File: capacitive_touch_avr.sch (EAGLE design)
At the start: 10 parts, among them J2 JACK-2.1MM

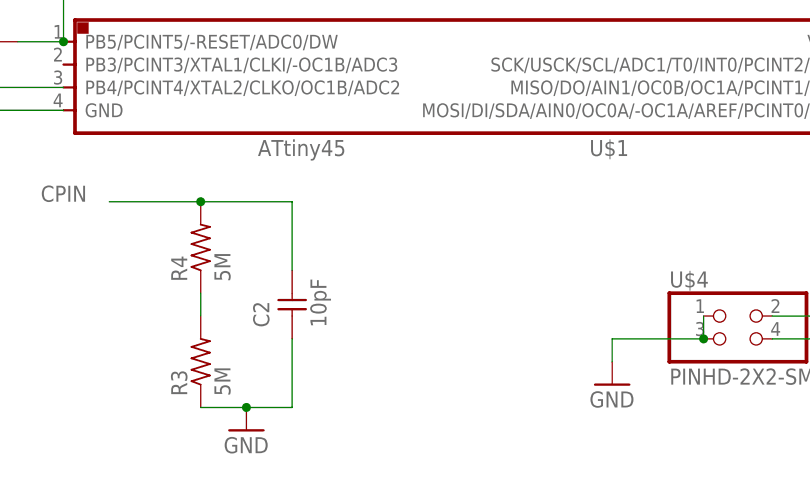
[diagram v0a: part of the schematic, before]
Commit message: Version 1. Touch pad + full wiring
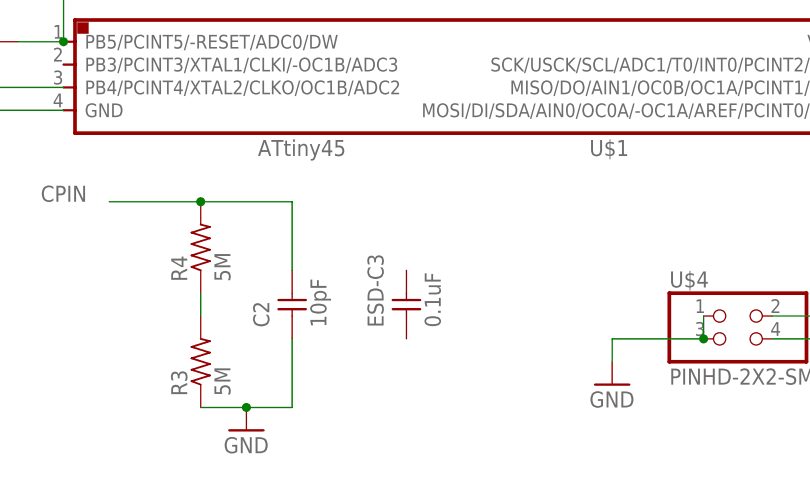
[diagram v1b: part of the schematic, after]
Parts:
- added ESD-C3: 0.1uF, fab:CAP-UNPOLARIZEDFAB
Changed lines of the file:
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@@
 <part name="P+7" library="supply1" library_urn="urn:adsk.eagle:library:371" deviceset="VCC" device=""/>
 <part name="J2" library="fab" deviceset="JACK-2.1MM" device=""/>
+<part name="ESD-C3" library="fab" deviceset="CAP-UNPOLARIZED" device="FAB" value="0.1uF"/>
 </parts>
 <sheets>
@@
 <instance part="P+7" gate="VCC" x="25.4" y="58.42" rot="R180"/>
 <instance part="J2" gate="G$1" x="27.94" y="73.66" rot="R90"/>
+<instance part="ESD-C3" gate="&gt;NAME" x="53.34" y="22.86" rot="R90"/>
 </instances>
 <busses>
